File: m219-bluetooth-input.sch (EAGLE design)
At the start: 68 parts, among them U1 SCREW-M2X8, U10 FX2-20S-1.27DS, U2 SCREW-M2X8, U3 NUT-M2-SELFLOCK, U4 NUT-M2-SELFLOCK, U5 FX2-20P-1.27DS, U6 SCREW-M2X8, U7 SCREW-M2X8, U8 NUT-M2-SELFLOCK, U9 NUT-M2-SELFLOCK

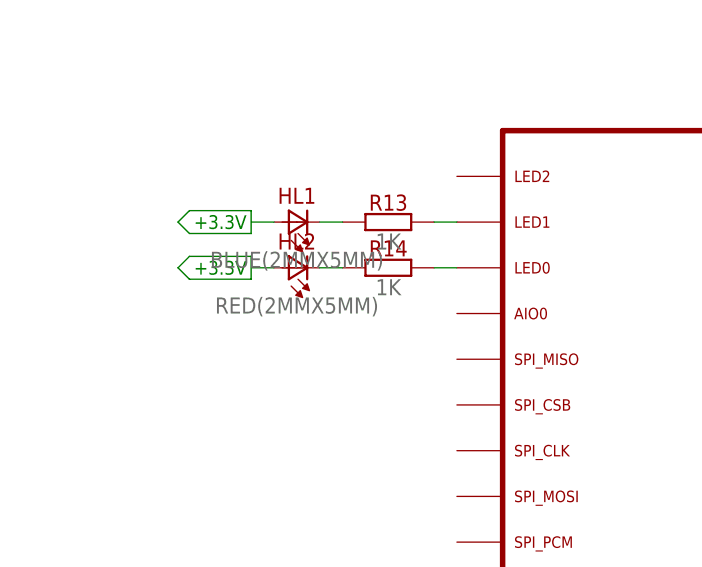
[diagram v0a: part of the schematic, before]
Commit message: M219a Routing
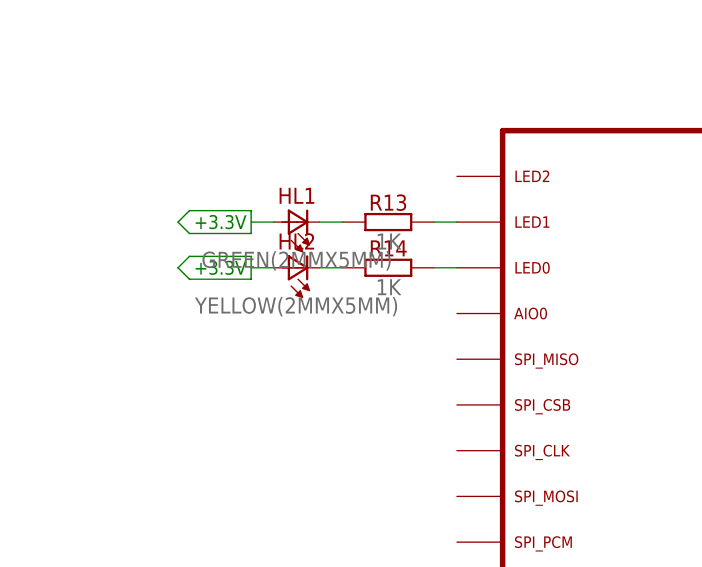
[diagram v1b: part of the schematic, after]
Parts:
- HL1: value BLUE(2MMX5MM) -> GREEN(2MMX5MM); device optoelectronics:BLUE(2MMX5MM) -> optoelectronics:GREEN(2MMX5MM)
- HL2: value RED(2MMX5MM) -> YELLOW(2MMX5MM); device optoelectronics:RED(2MMX5MM) -> optoelectronics:YELLOW(2MMX5MM)
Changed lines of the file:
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@@
 <part name="R13" library="resistors" deviceset="?" device="1K"/>
 <part name="R14" library="resistors" deviceset="?" device="1K"/>
-<part name="HL2" library="optoelectronics" deviceset="?(2MMX5MM)" device="RED" value="RED(2MMX5MM)"/>
-<part name="HL1" library="optoelectronics" deviceset="?(2MMX5MM)" device="BLUE" value="BLUE(2MMX5MM)"/>
+<part name="HL2" library="optoelectronics" deviceset="?(2MMX5MM)" device="YELLOW" value="YELLOW(2MMX5MM)"/>
+<part name="HL1" library="optoelectronics" deviceset="?(2MMX5MM)" device="GREEN" value="GREEN(2MMX5MM)"/>
 <part name="PWR1" library="supply" deviceset="+3.3V" device=""/>
 <part name="PWR2" library="supply" deviceset="+3.3V" device=""/>
